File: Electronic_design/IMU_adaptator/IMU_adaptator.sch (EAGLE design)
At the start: 8 parts, among them J1 CLM-110-02-XX-D

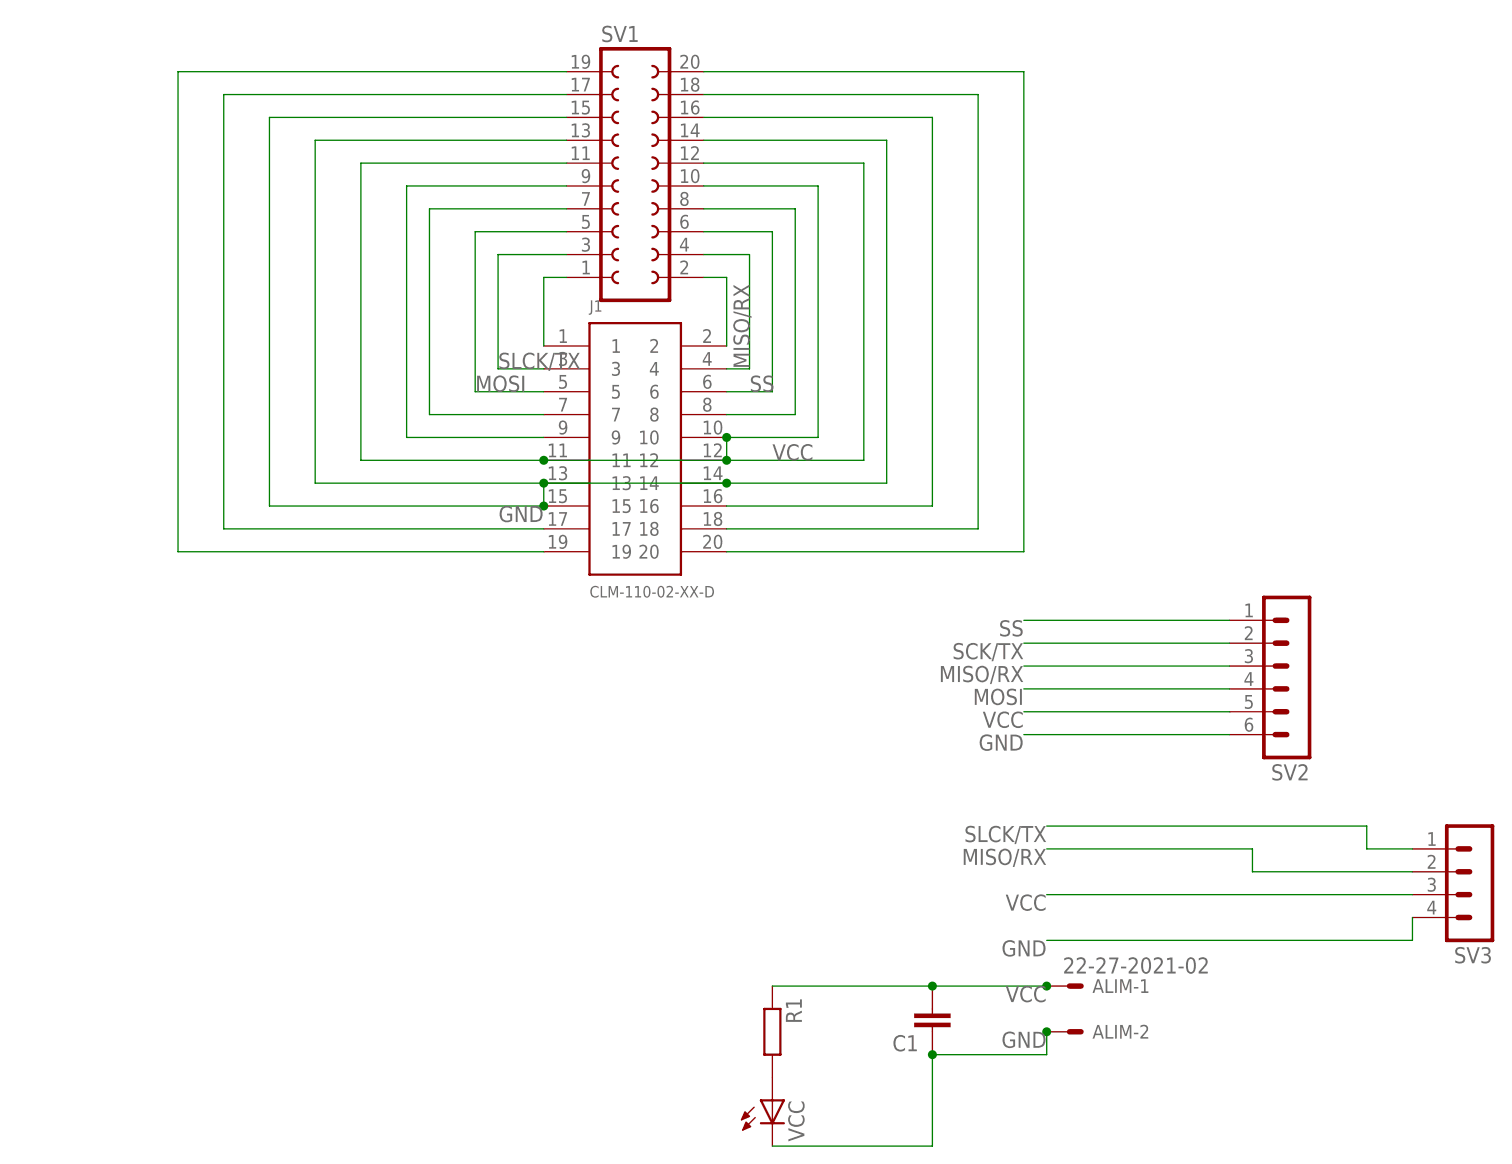
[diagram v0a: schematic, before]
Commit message: nouveau routage
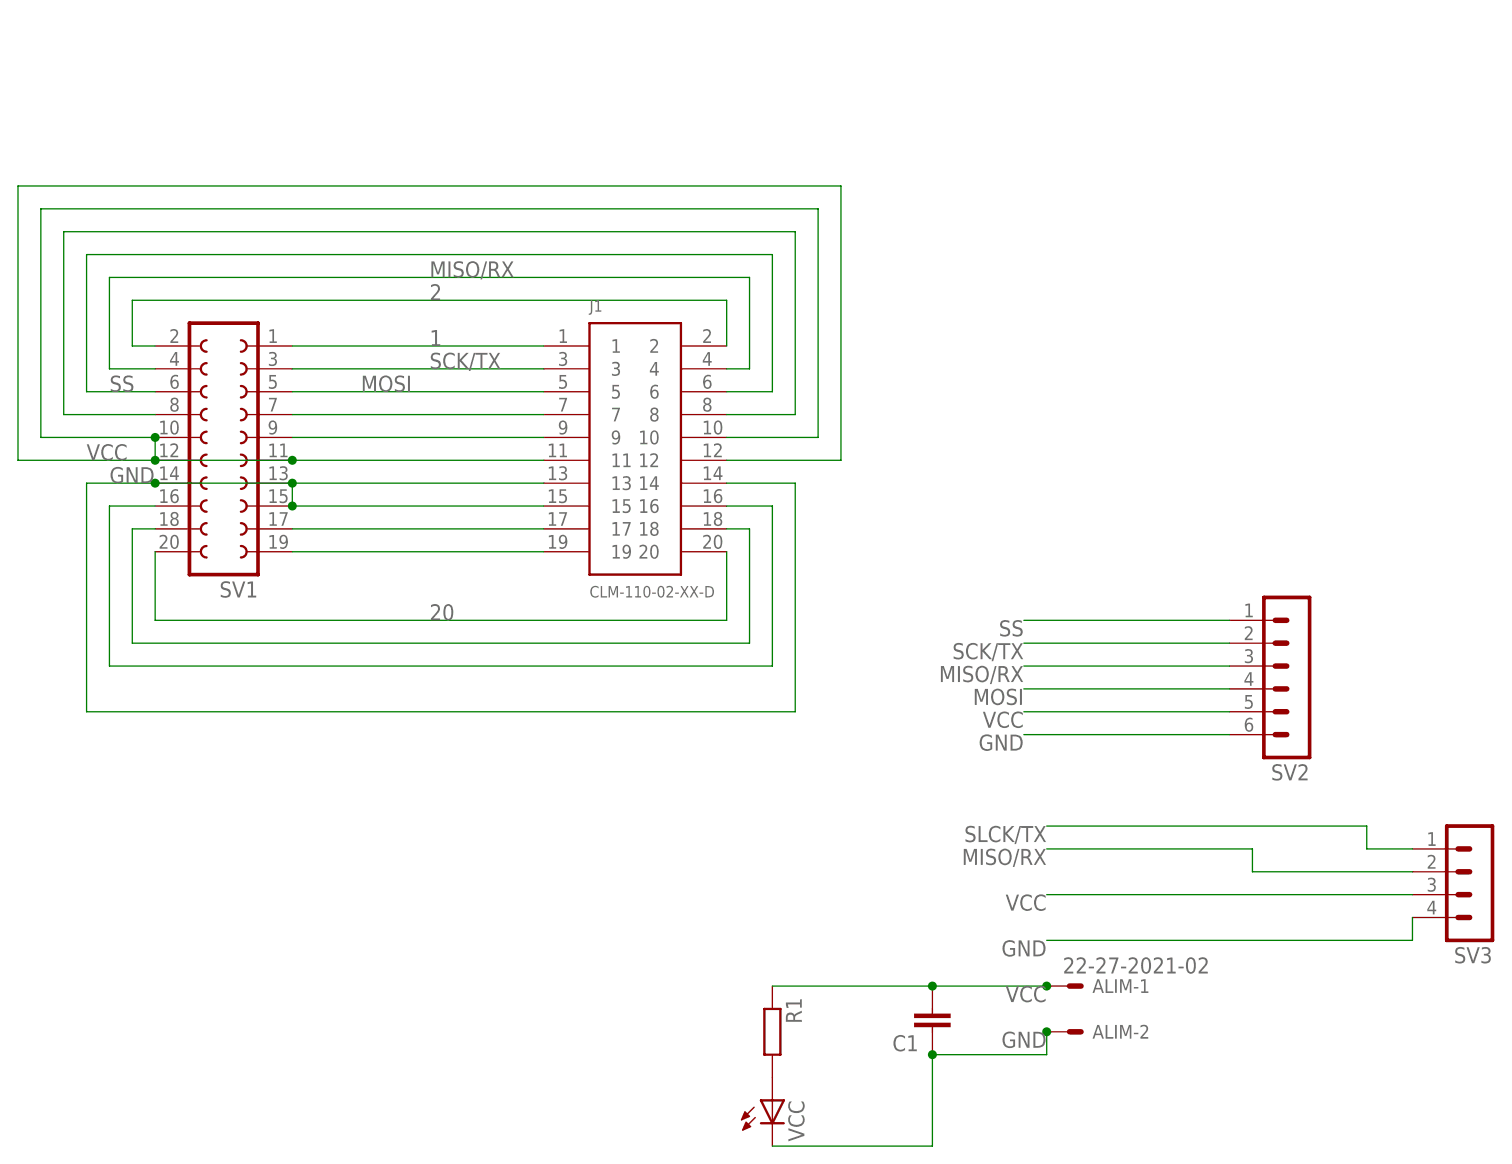
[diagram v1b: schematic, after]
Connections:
- net N$1 renamed 1
- net N$2 renamed 2
- net N$20 renamed 20
- net SCK/TX: now also J1.3, SV1.3
- net SLCK/TX: no longer J1.3, SV1.3
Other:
- moved on the sheet: SV1
